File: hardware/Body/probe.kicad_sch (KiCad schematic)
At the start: 6 parts, among them Q4 BC337

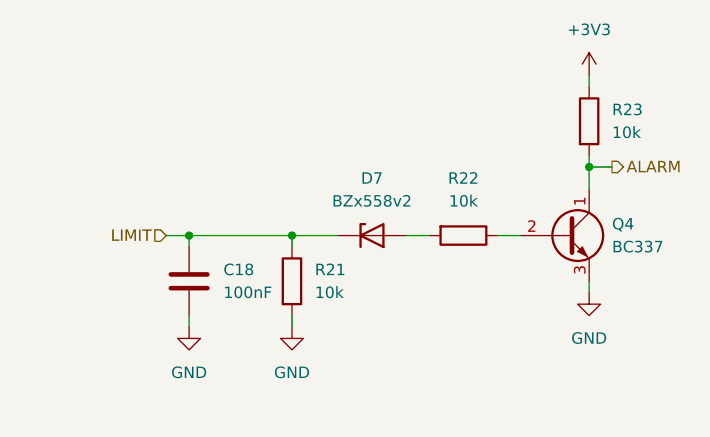
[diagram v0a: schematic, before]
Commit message: body
Signed-off-by: cukier <mauricio@krebs.com.br>
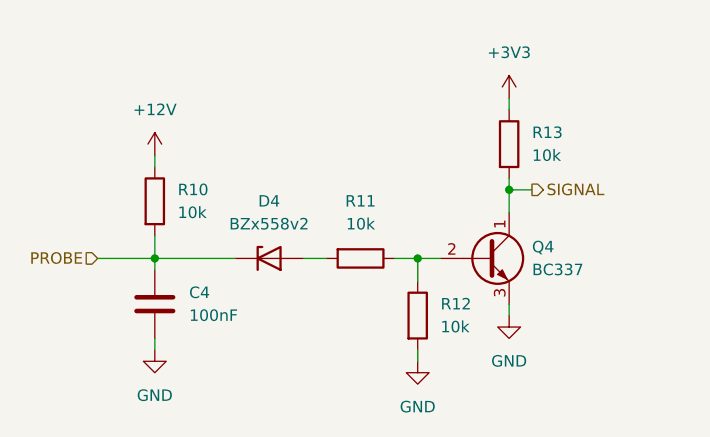
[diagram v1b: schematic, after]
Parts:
- removed C18: 100nF, Capacitor_SMD:C_1206_3216Metric, symbol Device:C
- removed D7: BZx558v2, Diode_SMD:D_MELF_Handsoldering, symbol Device:D_Zener
- removed R21, R22, R23: 10k, Resistor_SMD:R_1206_3216Metric, symbol Device:R
- added C4: 100nF, Capacitor_SMD:C_1206_3216Metric_Pad1.33x1.80mm_HandSolder, symbol Device:C
- added D4: BZx558v2, Diode_SMD:D_MELF_Handsoldering, symbol Device:D_Zener
- added R10, R11, R12, R13: 10k, Resistor_SMD:R_1206_3216Metric_Pad1.30x1.75mm_HandSolder, symbol Device:R
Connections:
- net +3V3: now also R13.1
- net GND: now also C4.2, R12.2
- net at Q4.2 (B): now also R11.1, R12.1
- net ALARM renamed SIGNAL
- net SIGNAL: now also R13.2
- new net: D4.2 (A), R11.2
- new net +12V: R10.1
- new net PROBE: C4.1, D4.1 (K), R10.2
